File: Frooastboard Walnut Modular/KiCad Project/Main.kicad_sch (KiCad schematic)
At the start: 214 parts, among them J10 F Row CS, J11 F Row SW, J15 F Row, J16 F Row USB, J17 Numpad, J8 Numpad CS, J9 Numpad SW, M2 Frooastboard_MM2040

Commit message: asign pieces
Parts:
- MX100, MX101, MX102, MX103, MX104, MX105, MX107, MX108, MX109, MX110, MX39, MX44, MX45, MX46, MX47, MX48, MX49, MX50, MX51, MX53, MX54, MX55, MX56, MX57, MX58, MX59, MX60, MX62, MX63, MX64, MX65, MX66, MX67, MX68, MX69, MX71, MX72, MX73, MX74, MX75, MX76, MX77, MX78, MX80, MX81, MX82, MX84, MX85, MX86, MX87, MX91, MX92, MX93, MX94, MX95, MX96, MX98, MX99: footprint (none) -> MX_Only:MXOnly-1U-NoLED
- MX106, MX42, MX43, MX52, MX61, MX79, MX88, MX97: footprint (none) -> MX_Only:MXOnly-1.25U-NoLED
- MX111, MX113: footprint (none) -> MX_Only:MXOnly-2.25U-NoLED
- MX112, MX40: footprint (none) -> MX_Only:MXOnly-1.5U-NoLED
- MX41: footprint (none) -> MX_Only:MXOnly-1.75U
- MX70: footprint (none) -> MX_Only:MXOnly-6.25U-ReversedStabilizers-NoLED
- MX83: footprint (none) -> MX_Only:MXOnly-2.75U-NoLED
- MX89: footprint (none) -> MX_Only:MXOnly-2U-NoLED
- MX90: footprint (none) -> MX_Only:MXOnly-ISO-ROTATED-NoLED-NoStabilizers
- R25: footprint (none) -> Resistor_SMD:R_0805_2012Metric

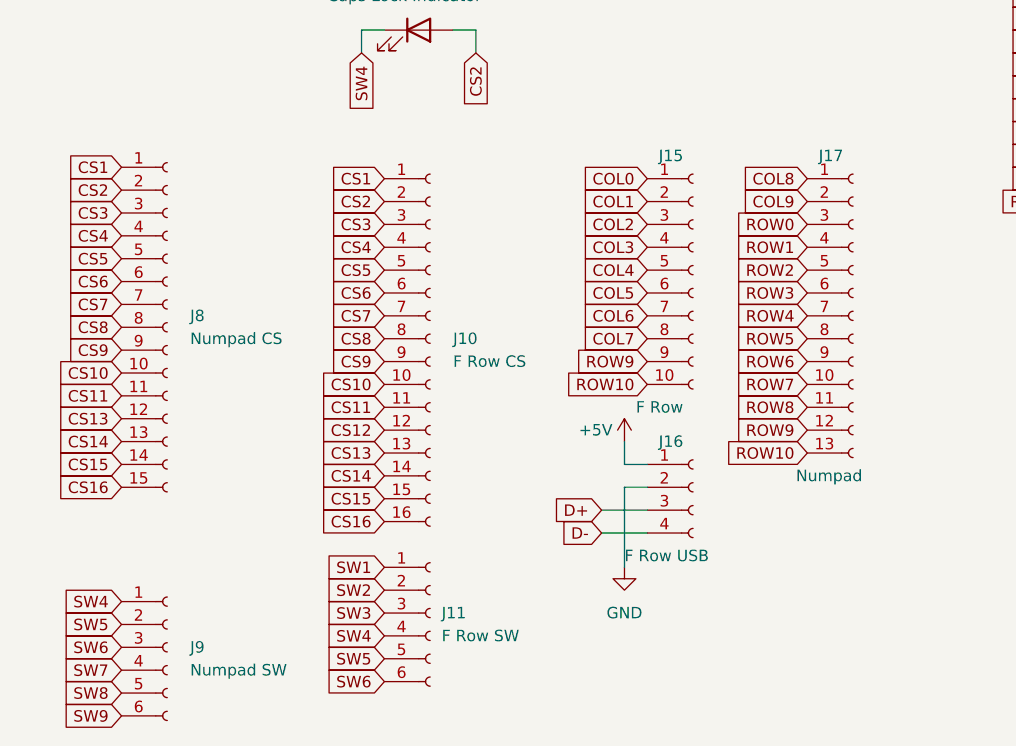
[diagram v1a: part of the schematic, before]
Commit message: more footprint changes
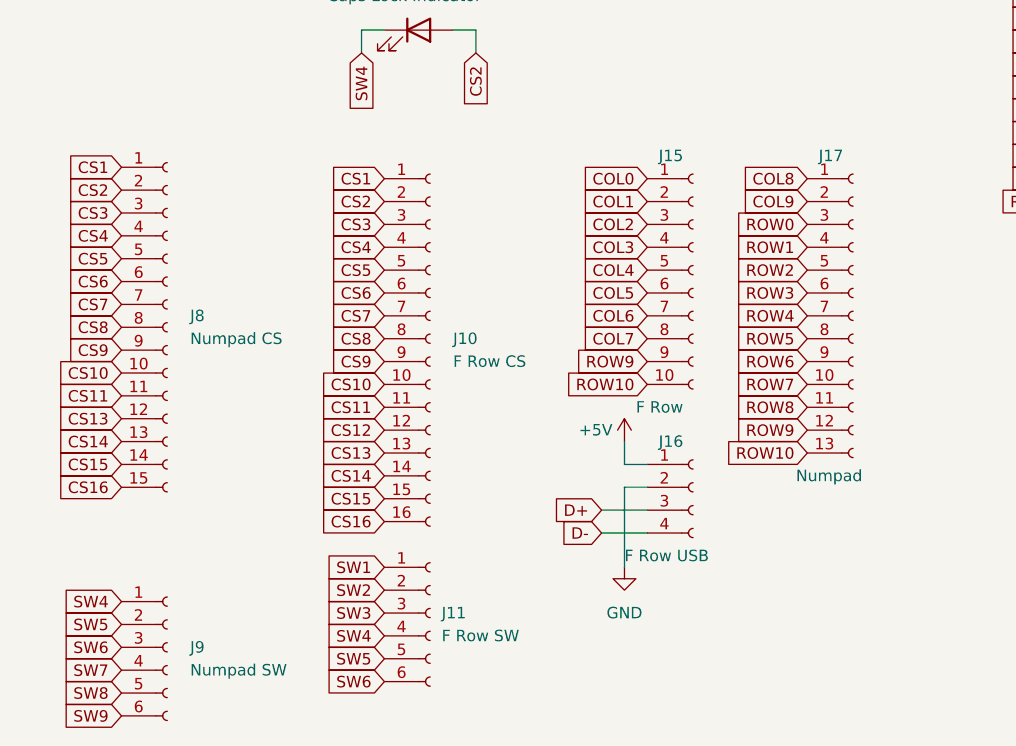
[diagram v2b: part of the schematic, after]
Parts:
- J10, J8: footprint Frooastboard Footprints:PinHeader_1x16_P1.27mm_Vertical -> Connector_PinHeader_1.27mm:PinHeader_1x16_P1.27mm_Vertical
- J11, J9: footprint Frooastboard Footprints:PinHeader_1x06_P1.27mm_Vertical -> Connector_PinHeader_1.27mm:PinHeader_1x06_P1.27mm_Vertical
- J15: footprint Frooastboard Footprints:PinHeader_1x10_P1.27mm_Vertical -> Connector_PinHeader_1.27mm:PinHeader_1x10_P1.27mm_Vertical
- J16: footprint Frooastboard Footprints:PinHeader_1x04_P1.27mm_Vertical -> Connector_PinHeader_1.27mm:PinHeader_1x04_P1.27mm_Vertical
- J17: footprint Frooastboard Footprints:PinHeader_1x13_P1.27mm_Vertical -> Connector_PinHeader_1.27mm:PinHeader_1x13_P1.27mm_Vertical
